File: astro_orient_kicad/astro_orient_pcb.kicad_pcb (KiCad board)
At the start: 2 copper layers, 72 x 49 mm, 45 parts, among them J1 BME260, J2 SWD_Tag_Connect, J3 USB-C_Receptacle, SW1 SW_SPST, U1 STM32F072CBTx, U2 AP2112K-3.3, U3 AP2112K-3.3, Y1 osc_crystal

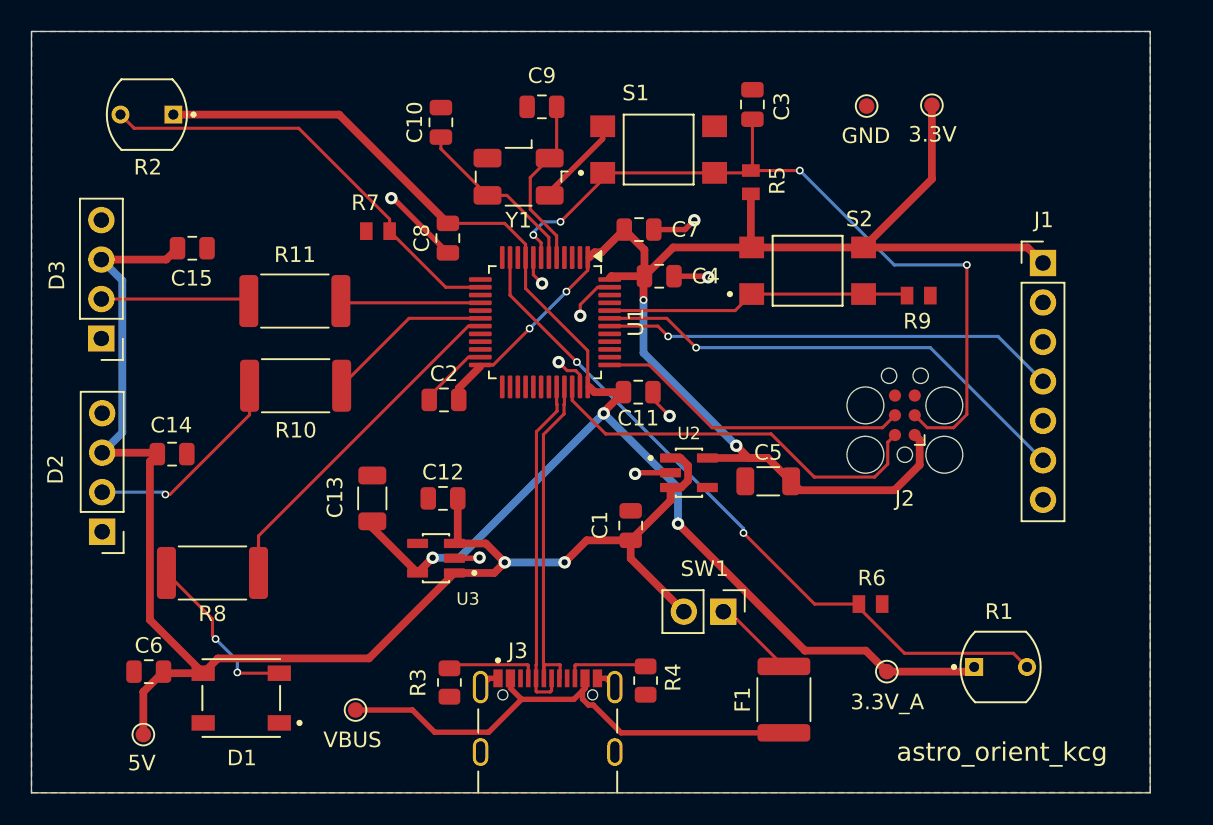
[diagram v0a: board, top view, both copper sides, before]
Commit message: last changes to PCB
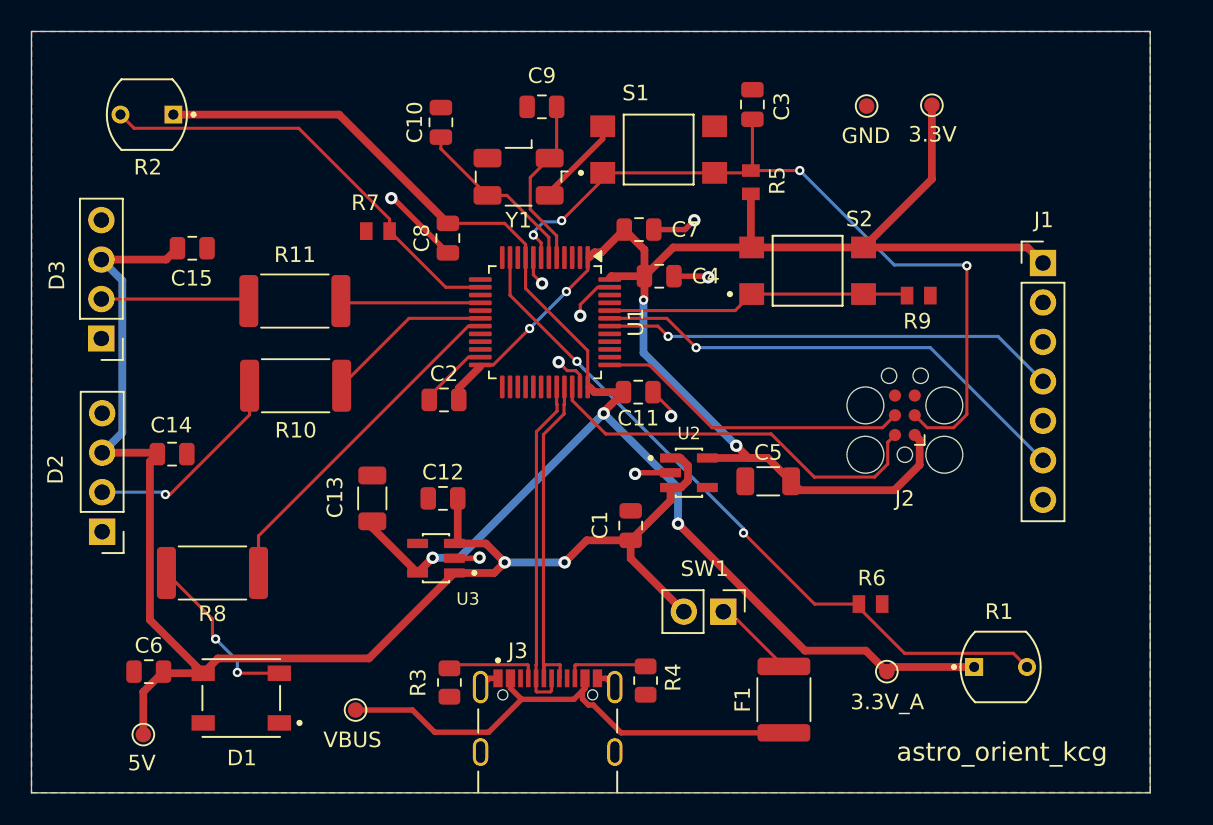
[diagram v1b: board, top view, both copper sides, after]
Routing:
- net GND: track 36.7 -> 37.3 mm
